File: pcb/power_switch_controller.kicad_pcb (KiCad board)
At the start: 2 copper layers, 118.1 x 54.6 mm, 37 parts, among them P1 PWR_JACK_2.5x5.5, P2 HEADER_01X03, P3 BNC_DOUBLE_RA, P4 HEADER_02X16, SW1 SPST_SERIES_M, U1 MAX6817, U2 TLE723X, U3 TLE723X

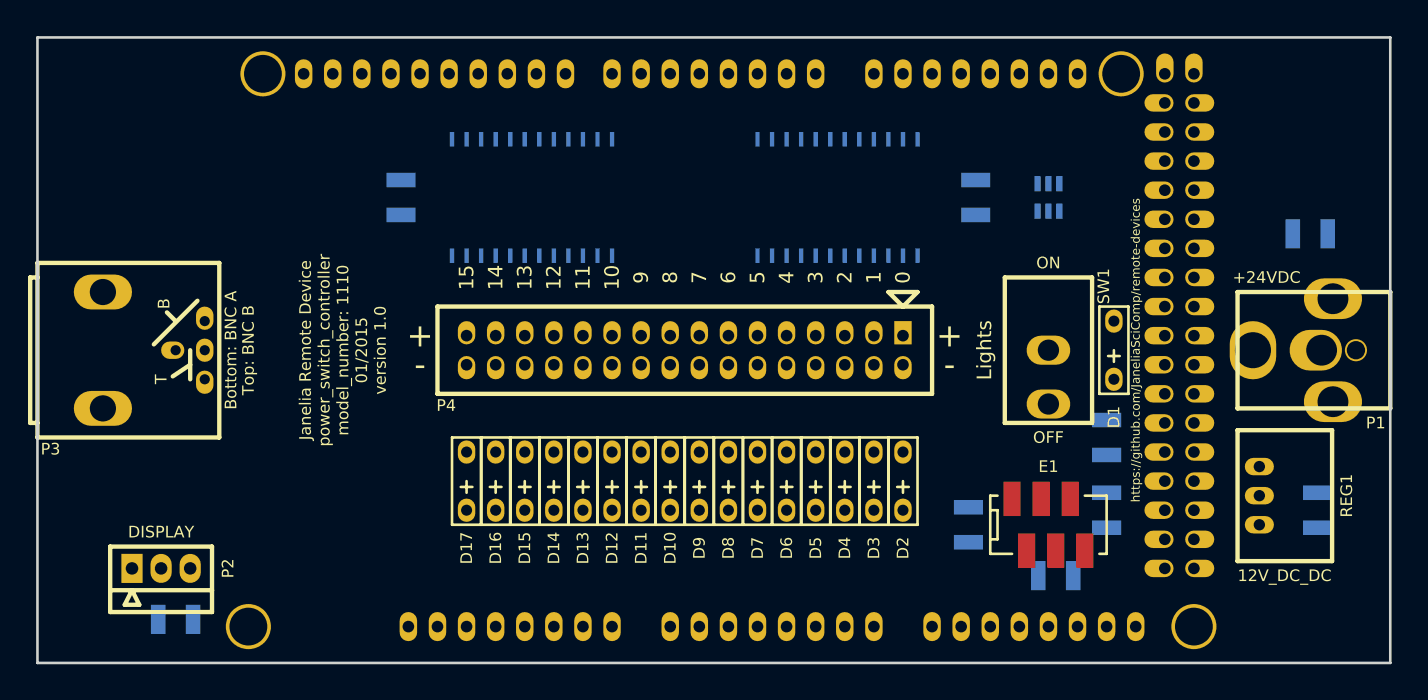
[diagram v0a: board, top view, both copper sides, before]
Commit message: Finished pcb version 1.0
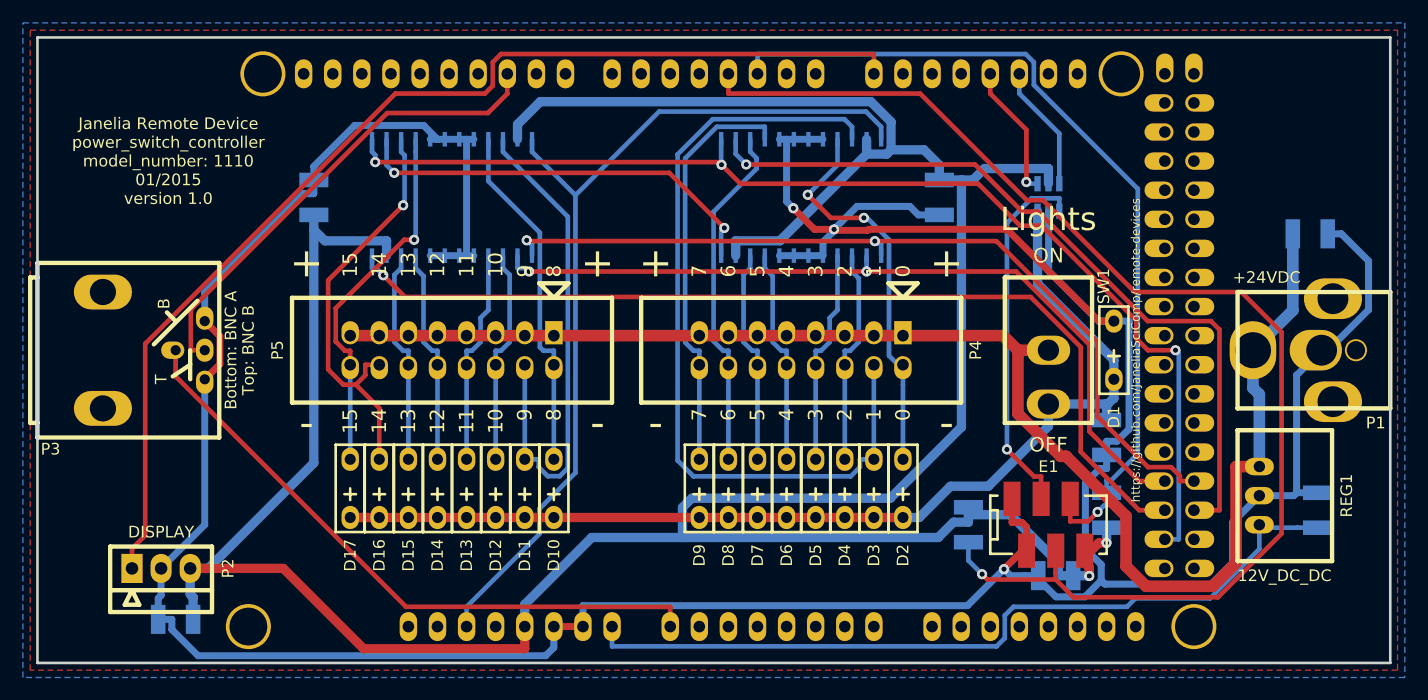
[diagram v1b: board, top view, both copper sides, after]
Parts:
- added P5: HEADER_02X08, power_switch_controller:HEADER_02x08, F.Cu at (129.5, 102.9)
- P4: value HEADER_02X16 -> HEADER_02X08; footprint power_switch_controller:HEADER_02x32 -> power_switch_controller:HEADER_02x08
- moved D11 10.2 mm to (135.9, 114.9)
- moved D10 10.2 mm to (138.4, 114.9)
- moved D12 10.2 mm to (133.3, 114.9)
- moved D13 10.2 mm to (130.8, 114.9)
- moved D14 10.2 mm to (128.3, 114.9)
- moved D16 10.2 mm to (123.2, 114.9)
- moved D17 10.2 mm to (120.7, 114.9)
- moved D15 10.2 mm to (125.7, 114.9)
- moved P4 10.2 mm to (160.0, 102.9)
- moved C6 7.62 mm to (117.5, 89.5)
- moved U3 6.99 mm to (129.5, 89.5)
- moved C5 3.17 mm to (172.1, 89.5)
- moved U2 3.17 mm to (160.0, 89.5)
- moved D2 0.64 mm to (168.9, 114.9)
- moved D3 0.64 mm to (166.4, 114.9)
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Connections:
- ARDUINO1 pad 10: (no net) -> /BNC_B
- ARDUINO1 pad 20B: /BNC_B -> (no net)
- ARDUINO1 pad 21B: /BNC_A -> (no net)
- ARDUINO1 pad A0: (no net) -> /BNC_A
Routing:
- net GND: track 0.00 -> 327.8 mm, vias 0 -> 3
- net +5V: track 0.00 -> 273.5 mm, vias 0 -> 2
- net VAA: track 0.00 -> 128.2 mm
- net /ENC_B: track 0.00 -> 111.3 mm, vias 0 -> 1
- net /SCK: track 0.00 -> 99.8 mm, vias 0 -> 3
- net /TX3: track 0.00 -> 97.1 mm
- net /LED_PWR: track 0.00 -> 92.6 mm
- net /MISO: track 0.00 -> 84.4 mm, vias 0 -> 1
- net /RST: track 0.00 -> 79.4 mm
- net /ENC_A: track 0.00 -> 75.7 mm, vias 0 -> 1
- net /CS: track 0.00 -> 74.4 mm, vias 0 -> 2
- net /OUT1: track 0.00 -> 71.6 mm
- net /IN: track 0.00 -> 71.1 mm, vias 0 -> 2
- net /V_IN: track 0.00 -> 70.1 mm
- net /MOSI: track 0.00 -> 67.9 mm, vias 0 -> 1
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- added copper zone on B.Cu, net GND
- added copper zone on F.Cu, net VAA
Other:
- net class SUPERPOWER: trace_width 1.2192 -> 1.016
- board text added: "+"
- board text added: "-"
- board text added: "0"
- board text added: "1"
- board text added: "10"
- board text added: "11"
- board text added: "12"
- board text added: "13"
- board text added: "14"
- board text added: "15"
- board text added: "2"
- board text added: "3"
- board text added: "4"
- board text added: "5"
- board text added: "6"
- board text added: "7"
- board text added: "8"
- board text added: "9"
